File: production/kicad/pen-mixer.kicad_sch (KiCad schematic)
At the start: 28 parts, among them J1 USB-C 16P, J2 BAT, U1 ISP1807-LR, U2 LSM6DS3TR-C, U3 MCP73831T-2ACI/OT, U4 TPS7A0533PDBV

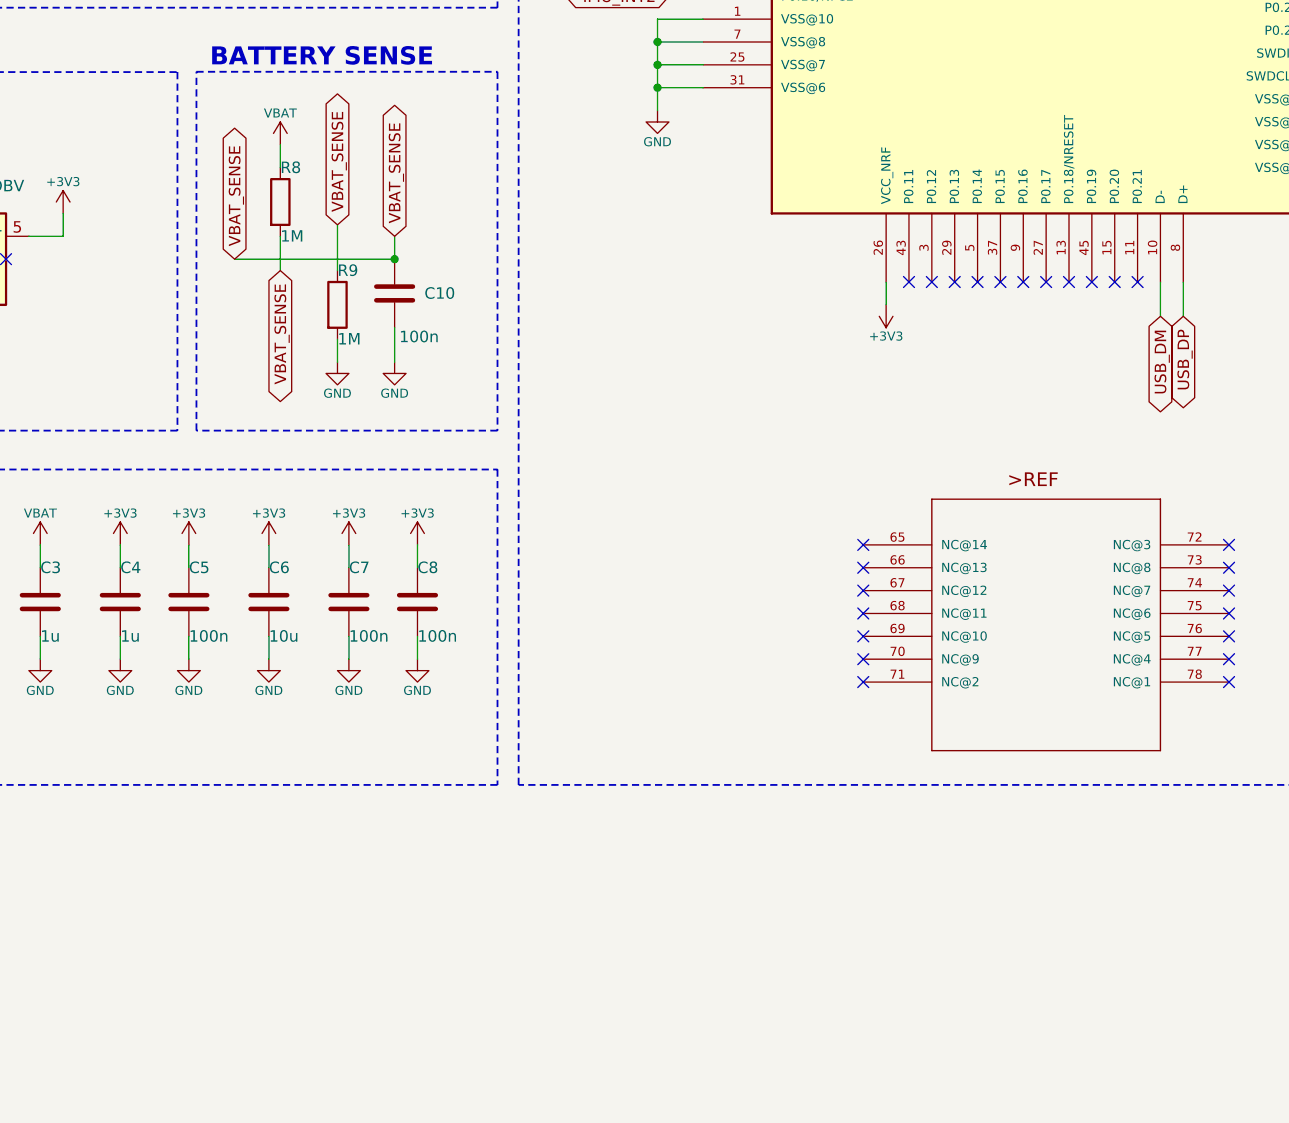
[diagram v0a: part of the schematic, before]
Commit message: add v21 hardware
Claude-Session: https://claude.ai/code/session_01RCYT2QSY7BVZDeTyE9KrC4
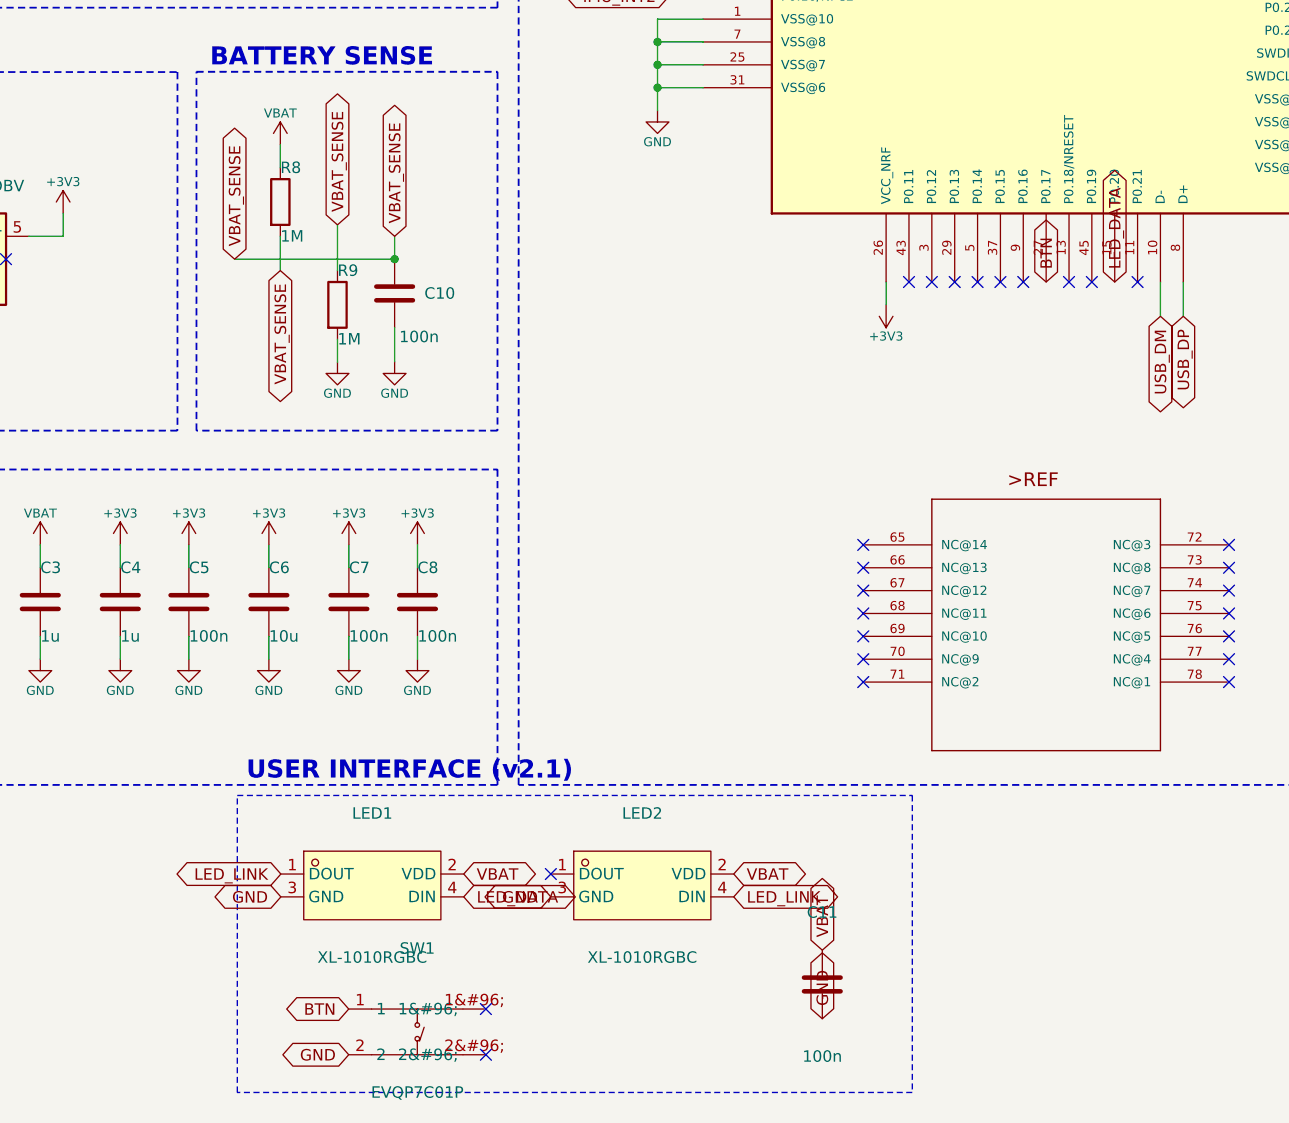
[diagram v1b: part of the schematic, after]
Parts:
- added C11: 100n, Capacitor_SMD:C_0402_1005Metric, symbol Device:C
- added LED1, LED2: XL-1010RGBC, pen-mixer:LED-SMD_4P-L1.0-W1.0-TL_XL-1010RGBC-WS2812B, symbol v21:XL-1010RGBC
- added SW1: EVQP7C01P, pen-mixer:SW-SMD_EVQP7C01P, symbol v21:EVQP7C01P
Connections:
- net GND: now also C11.2, LED1.3 (GND), LED2.3 (GND), SW1.2
- net VBAT: now also C11.1, LED1.2 (VDD), LED2.2 (VDD)
- net LED_DATA: now reaches U1.15 (P0.20)
- net LED_DATA: now also LED1.4 (DIN)
- net BTN: now reaches U1.27 (P0.17)
- net BTN: now also SW1.1
- new net LED_LINK: LED1.1 (DOUT), LED2.4 (DIN)
- no-connect marks 60 -> 61
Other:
- note added: "USER INTERFACE (v2.1)"
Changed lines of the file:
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@@
 	)
 	(no_connect
-		(at 237.49 107.95)
-	)
-	(no_connect
 		(at 208.28 33.02)
 	)
@@
 	)
 	(no_connect
-		(at 229.87 107.95)
-	)
-	(no_connect
 		(at 114.3 105.41)
 	)
@@
 		(color 0 0 0 0)
 	)
+	(symbol
+		(lib_id "v21:XL-1010RGBC")
+		(at 155 175 0)
+		(unit 1)
+		(body_style 1)
+		(exclude_from_sim no)
+		(in_bom yes)
+		(on_board yes)
+		(dnp no)
+		(property "Reference" "LED1" (at 155 167 0)  (effects (font (size 1.27 1.27))))
+		(property "Value" "XL-1010RGBC" (at 155 183 0)  (effects (font (size 1.27 1.27))))
+		(property "Footprint" "pen-mixer:LED-SMD_4P-L1.0-W1.0-TL_XL-1010RGBC-WS2812B" (at 155 175 0) (hide yes) (effects (font (size 1.27 1.27))))
+		(property "Datasheet" "" (at 155 175 0) (hide yes) (effects (font (size 1.27 1.27))))
+		(property "MPN" "XL-1010RGBC-2812B" (at 155 175 0) (hide yes) (effects (font (size 1.27 1.27))))
+		(property "Manufacturer" "XINGLIGHT" (at 155 175 0) (hide yes) (effects (font (size 1.27 1.27))))
+		(property "LCSC" "C5349953" (at 155 175 0) (hide yes) (effects (font (size 1.27 1.27))))
+		(property "BOM Comments" "battery level indicator" (at 155 175 0) (hide yes) (effects (font (size 1.27 1.27))))
+		(instances (project "pen-mixer" (path "/0684e67f-dde5-4049-a068-2c0d069dd8c7" (reference "LED1") (unit 1))))
+	)
+	(symbol
+		(lib_id "v21:XL-1010RGBC")
+		(at 185 175 0)
+		(unit 1)
+		(body_style 1)
+		(exclude_from_sim no)
+		(in_bom yes)
+		(on_board yes)
+		(dnp no)
+		(property "Reference" "LED2" (at 185 167 0)  (effects (font (size 1.27 1.27))))
+		(property "Value" "XL-1010RGBC" (at 185 183 0)  (effects (font (size 1.27 1.27))))
+		(property "Footprint" "pen-mixer:LED-SMD_4P-L1.0-W1.0-TL_XL-1010RGBC-WS2812B" (at 185 175 0) (hide yes) (effects (font (size 1.27 1.27))))
+		(property "Datasheet" "" (at 185 175 0) (hide yes) (effects (font (size 1.27 1.27))))
+		(property "MPN" "XL-1010RGBC-2812B" (at 185 175 0) (hide yes) (effects (font (size 1.27 1.27))))
+		(property "Manufacturer" "XINGLIGHT" (at 185 175 0) (hide yes) (effects (font (size 1.27 1.27))))
+		(property "LCSC" "C5349953" (at 185 175 0) (hide yes) (effects (font (size 1.27 1.27))))
+		(property "BOM Comments" "bluetooth status indicator" (at 185 175 0) (hide yes) (effects (font (size 1.27 1.27))))
+		(instances (project "pen-mixer" (path "/0684e67f-dde5-4049-a068-2c0d069dd8c7" (reference "LED2") (unit 1))))
+	)
+	(symbol
+		(lib_id "v21:EVQP7C01P")
+		(at 160 190 0)
+		(unit 1)
+		(body_style 1)
+		(exclude_from_sim no)
+		(in_bom yes)
+		(on_board yes)
+		(dnp no)
+		(property "Reference" "SW1" (at 160 182 0)  (effects (font (size 1.27 1.27))))
+		(property "Value" "EVQP7C01P" (at 160 198 0)  (effects (font (size 1.27 1.27))))
+		(property "Footprint" "pen-mixer:SW-SMD_EVQP7C01P" (at 160 190 0) (hide yes) (effects (font (size 1.27 1.27))))
+		(property "Datasheet" "" (at 160 190 0) (hide yes) (effects (font (size 1.27 1.27))))
+		(property "MPN" "EVQP7C01P" (at 160 190 0) (hide yes) (effects (font (size 1.27 1.27))))
+		(property "Manufacturer" "PANASONIC" (at 160 190 0) (hide yes) (effects (font (size 1.27 1.27))))
+		(property "LCSC" "C388883" (at 160 190 0) (hide yes) (effects (font (size 1.27 1.27))))
+		(property "BOM Comments" "power and pairing button, side actuated" (at 160 190 0) (hide yes) (effects (font (size 1.27 1.27))))
+		(instances (project "pen-mixer" (path "/0684e67f-dde5-4049-a068-2c0d069dd8c7" (reference "SW1") (unit 1))))
+	)
+	(symbol
+		(lib_id "Device:C")
+		(at 205 186 0)
+		(unit 1)
+		(body_style 1)
+		(exclude_from_sim no)
+		(in_bom yes)
+		(on_board yes)
+		(dnp no)
+		(property "Reference" "C11" (at 205 178 0)  (effects (font (size 1.27 1.27))))
+		(property "Value" "100n" (at 205 194 0)  (effects (font (size 1.27 1.27))))
+		(property "Footprint" "Capacitor_SMD:C_0402_1005Metric" (at 205 186 0) (hide yes) (effects (font (size 1.27 1.27))))
+		(property "Datasheet" "" (at 205 186 0) (hide yes) (effects (font (size 1.27 1.27))))
+		(property "MPN" "CL05B104KO5NNNC" (at 205 186 0) (hide yes) (effects (font (size 1.27 1.27))))
+		(property "Manufacturer" "Samsung Electro-Mechanics" (at 205 186 0) (hide yes) (effects (font (size 1.27 1.27))))
+		(property "LCSC" "C1525" (at 205 186 0) (hide yes) (effects (font (size 1.27 1.27))))
+		(instances (project "pen-mixer" (path "/0684e67f-dde5-4049-a068-2c0d069dd8c7" (reference "C11") (unit 1))))
+	)
+	(global_label "LED_LINK"
+		(shape bidirectional)
+		(at 144.84 173.73 180)
+		(fields_autoplaced yes)
+		(effects (font (size 1.27 1.27)) (justify right))
+		(property "Intersheetrefs" "${INTERSHEET_REFS}" (at 144.84 173.73 0) (hide yes) (show_name no) (do_not_autoplace no) (effects (font (size 1.27 1.27))))
+	)
+	(global_label "GND"
+		(shape bidirectional)
+		(at 144.84 176.27 180)
+		(fields_autoplaced yes)
+		(effects (font (size 1.27 1.27)) (justify right))
+		(property "Intersheetrefs" "${INTERSHEET_REFS}" (at 144.84 176.27 0) (hide yes) (show_name no) (do_not_autoplace no) (effects (font (size 1.27 1.27))))
+	)
+	(global_label "VBAT"
+		(shape bidirectional)
+		(at 165.16 173.73 0)
+		(fields_autoplaced yes)
+		(effects (font (size 1.27 1.27)) (justify left))
+		(property "Intersheetrefs" "${INTERSHEET_REFS}" (at 165.16 173.73 0) (hide yes) (show_name no) (do_not_autoplace no) (effects (font (size 1.27 1.27))))
+	)
+	(global_label "LED_DATA"
+		(shape bidirectional)
+		(at 165.16 176.27 0)
+		(fields_autoplaced yes)
+		(effects (font (size 1.27 1.27)) (justify left))
+		(property "Intersheetrefs" "${INTERSHEET_REFS}" (at 165.16 176.27 0) (hide yes) (show_name no) (do_not_autoplace no) (effects (font (size 1.27 1.27))))
+	)
+	(no_connect
+		(at 174.84 173.73)
+	)
+	(global_label "GND"
+		(shape bidirectional)
+		(at 174.84 176.27 180)
+		(fields_autoplaced yes)
+		(effects (font (size 1.27 1.27)) (justify right))
+		(property "Intersheetrefs" "${INTERSHEET_REFS}" (at 174.84 176.27 0) (hide yes) (show_name no) (do_not_autoplace no) (effects (font (size 1.27 1.27))))
+	)
+	(global_label "VBAT"
+		(shape bidirectional)
+		(at 195.16 173.73 0)
+		(fields_autoplaced yes)
+		(effects (font (size 1.27 1.27)) (justify left))
+		(property "Intersheetrefs" "${INTERSHEET_REFS}" (at 195.16 173.73 0) (hide yes) (show_name no) (do_not_autoplace no) (effects (font (size 1.27 1.27))))
+	)
+	(global_label "LED_LINK"
+		(shape bidirectional)
+		(at 195.16 176.27 0)
+		(fields_autoplaced yes)
+		(effects (font (size 1.27 1.27)) (justify left))
+		(property "Intersheetrefs" "${INTERSHEET_REFS}" (at 195.16 176.27 0) (hide yes) (show_name no) (do_not_autoplace no) (effects (font (size 1.27 1.27))))
+	)
+	(global_label "BTN"
+		(shape bidirectional)
+		(at 152.38 188.73 180)
+		(fields_autoplaced yes)
+		(effects (font (size 1.27 1.27)) (justify right))
+		(property "Intersheetrefs" "${INTERSHEET_REFS}" (at 152.38 188.73 0) (hide yes) (show_name no) (do_not_autoplace no) (effects (font (size 1.27 1.27))))
+	)
+	(global_label "GND"
+		(shape bidirectional)
+		(at 152.38 193.81 180)
+		(fields_autoplaced yes)
+		(effects (font (size 1.27 1.27)) (justify right))
+		(property "Intersheetrefs" "${INTERSHEET_REFS}" (at 152.38 193.81 0) (hide yes) (show_name no) (do_not_autoplace no) (effects (font (size 1.27 1.27))))
+	)
+	(no_connect
+		(at 167.62 188.73)
+	)
+	(no_connect
+		(at 167.62 193.81)
+	)
+	(global_label "VBAT"
+		(shape bidirectional)
+		(at 205 182.19 90)
+		(fields_autoplaced yes)
+		(effects (font (size 1.27 1.27)) (justify left))
+		(property "Intersheetrefs" "${INTERSHEET_REFS}" (at 205 182.19 0) (hide yes) (show_name no) (do_not_autoplace no) (effects (font (size 1.27 1.27))))
+	)
+	(global_label "GND"
+		(shape bidirectional)
+		(at 205 189.81 270)
+		(fields_autoplaced yes)
+		(effects (font (size 1.27 1.27)) (justify left))
+		(property "Intersheetrefs" "${INTERSHEET_REFS}" (at 205 189.81 0) (hide yes) (show_name no) (do_not_autoplace no) (effects (font (size 1.27 1.27))))
+	)
+	(global_label "LED_DATA"
+		(shape bidirectional)
+		(at 237.49 107.95 270)
+		(fields_autoplaced yes)
+		(effects (font (size 1.27 1.27)) (justify left))
+		(property "Intersheetrefs" "${INTERSHEET_REFS}" (at 237.49 107.95 0) (hide yes) (show_name no) (do_not_autoplace no) (effects (font (size 1.27 1.27))))
+	)
+	(global_label "BTN"
+		(shape bidirectional)
+		(at 229.87 107.95 270)
+		(fields_autoplaced yes)
+		(effects (font (size 1.27 1.27)) (justify left))
+		(property "Intersheetrefs" "${INTERSHEET_REFS}" (at 229.87 107.95 0) (hide yes) (show_name no) (do_not_autoplace no) (effects (font (size 1.27 1.27))))
+	)
+	(rectangle
+		(start 140 165)
+		(end 215 198)
+		(stroke (width 0.1524) (type dash) (color 0 0 194 1))
+		(fill (type none))
+	)
+	(text "USER INTERFACE (v2.1)"
+		(exclude_from_sim no)
+		(at 141 163.5 0)
+		(effects (font (size 2 2) (bold yes) (color 0 0 194 1)) (justify left bottom))
+	)
 	(sheet_instances
